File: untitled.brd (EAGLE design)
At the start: 100 x 60 mm, 46 parts, among them IC1 LM393N, J1 61300311121, Q1 FQPF10N60C, Q2 s8550, Q3 s8550, Q4 s8550, T3 s8050

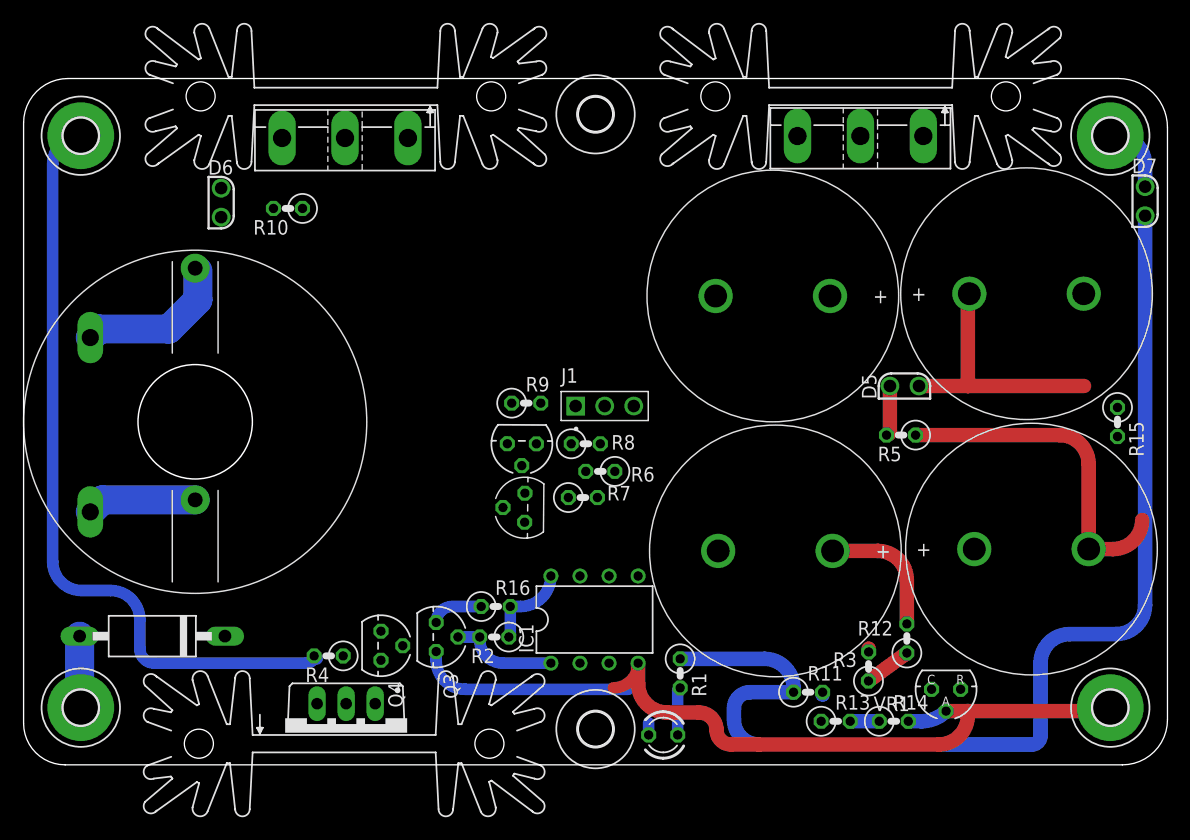
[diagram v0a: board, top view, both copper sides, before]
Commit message: add
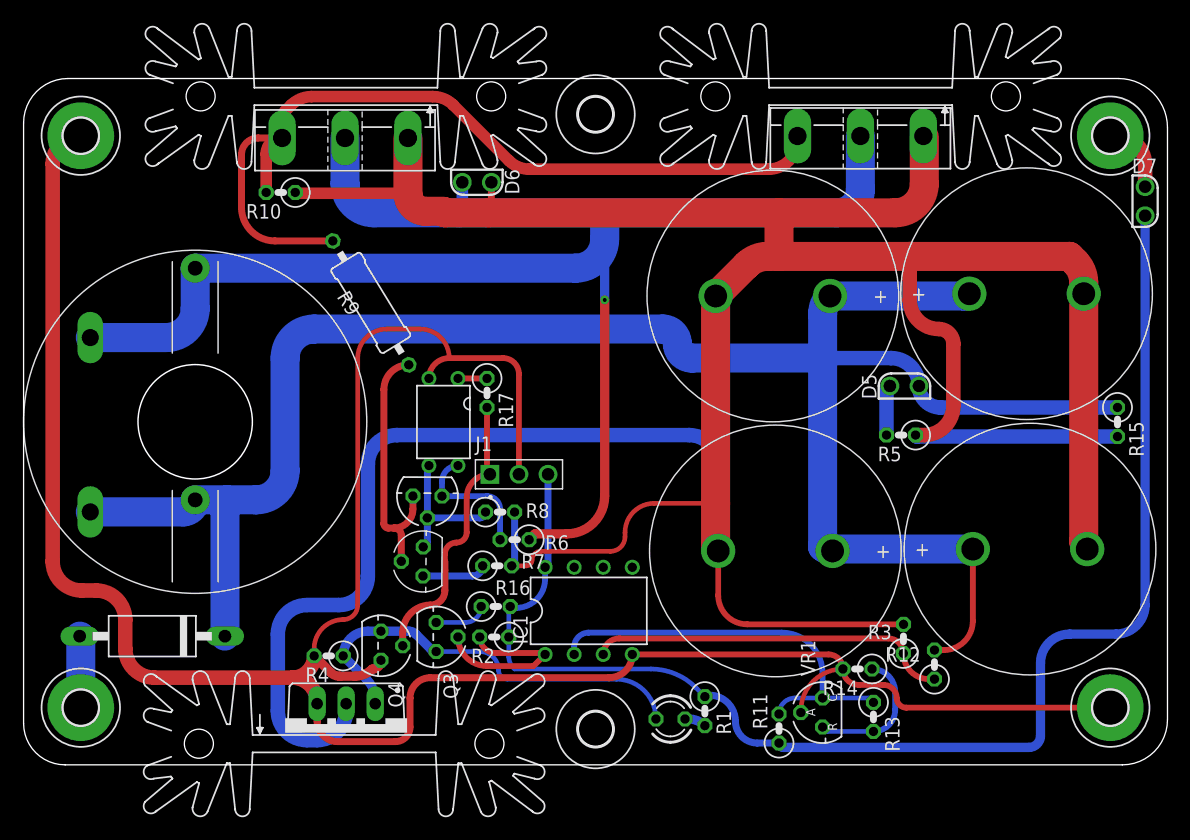
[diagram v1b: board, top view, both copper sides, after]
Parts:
- added OK1: SFH618A-4, optocoupler:DIP4
- added R17: 10k, rcl:0207/2V
- R6: value 10k -> 100k
- R9: device rcl:0207/2V -> rcl:0309/12
- moved D6 22.4 mm to (39.6, 50.9), turned to 270 degrees
- moved R9 16.2 mm to (30.4, 40.4), turned to 121.5 degrees
- moved VR1 11.0 mm to (69.8, 4.57), turned to 90 degrees
- moved T3 10.1 mm to (34.9, 17.8)
- moved R8 9.58 mm to (41.7, 22.1)
- moved R7 9.58 mm to (41.4, 17.4)
- moved J1 9.58 mm to (43.3, 25.4)
- moved R6 9.58 mm to (42.9, 19.7)
- moved Q2 9.44 mm to (35.3, 23.5)
- moved R14 5.57 mm to (72.9, 8.38), turned to 180 degrees
- moved R11 4.07 mm to (66.0, 3.17), turned to 90 degrees
- moved R1 3.95 mm to (59.6, 4.70)
- moved R3 3.89 mm to (76.9, 11.0)
- moved R12 3.32 mm to (79.6, 8.76)
- moved R13 3.32 mm to (74.3, 4.19), turned to 270 degrees
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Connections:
- new net N$12: OK1.1, R17.1
- new net N$14: OK1.3, Q2.2, R8.1, T3.1
- net BT+: no longer R6.1
- net BT-: now also OK1.2; no longer R7.2, R8.2
- net CIN: now also R17.2; no longer Q2.2, R8.1, T3.1
- net N$11: now also OK1.4
- net N$4: now also R6.1
- net N$8: now also R7.2, R8.2
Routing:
- net N$8: track 29.6 -> 311.8 mm
- net UC: track 43.6 -> 175.7 mm
- net N$4: track 13.3 -> 142.0 mm, vias 0 -> 1
- net BT-: track 122.2 -> 217.3 mm
- net SWITCH: track 0.00 -> 74.6 mm
- net N$5: track 0.22 -> 35.5 mm
- net CVO: track 4.15 -> 31.0 mm
- net CIN: track 0.00 -> 24.9 mm
- net N$9: track 0.00 -> 22.5 mm
- net CHARGE: track 19.7 -> 36.9 mm
- net BT+: track 105.2 -> 120.0 mm
- net N$14: track 0.00 -> 12.6 mm
- net N$11: track 0.00 -> 11.5 mm
- net N$7: track 2.54 -> 11.7 mm
- net N$1: track 9.22 -> 15.4 mm
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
